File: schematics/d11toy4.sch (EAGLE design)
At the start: 15 parts, among them J1 usb, J2 strip, SW1 SPST_TACT-KMR2, U3 XC6206P332MR-G-SOT23

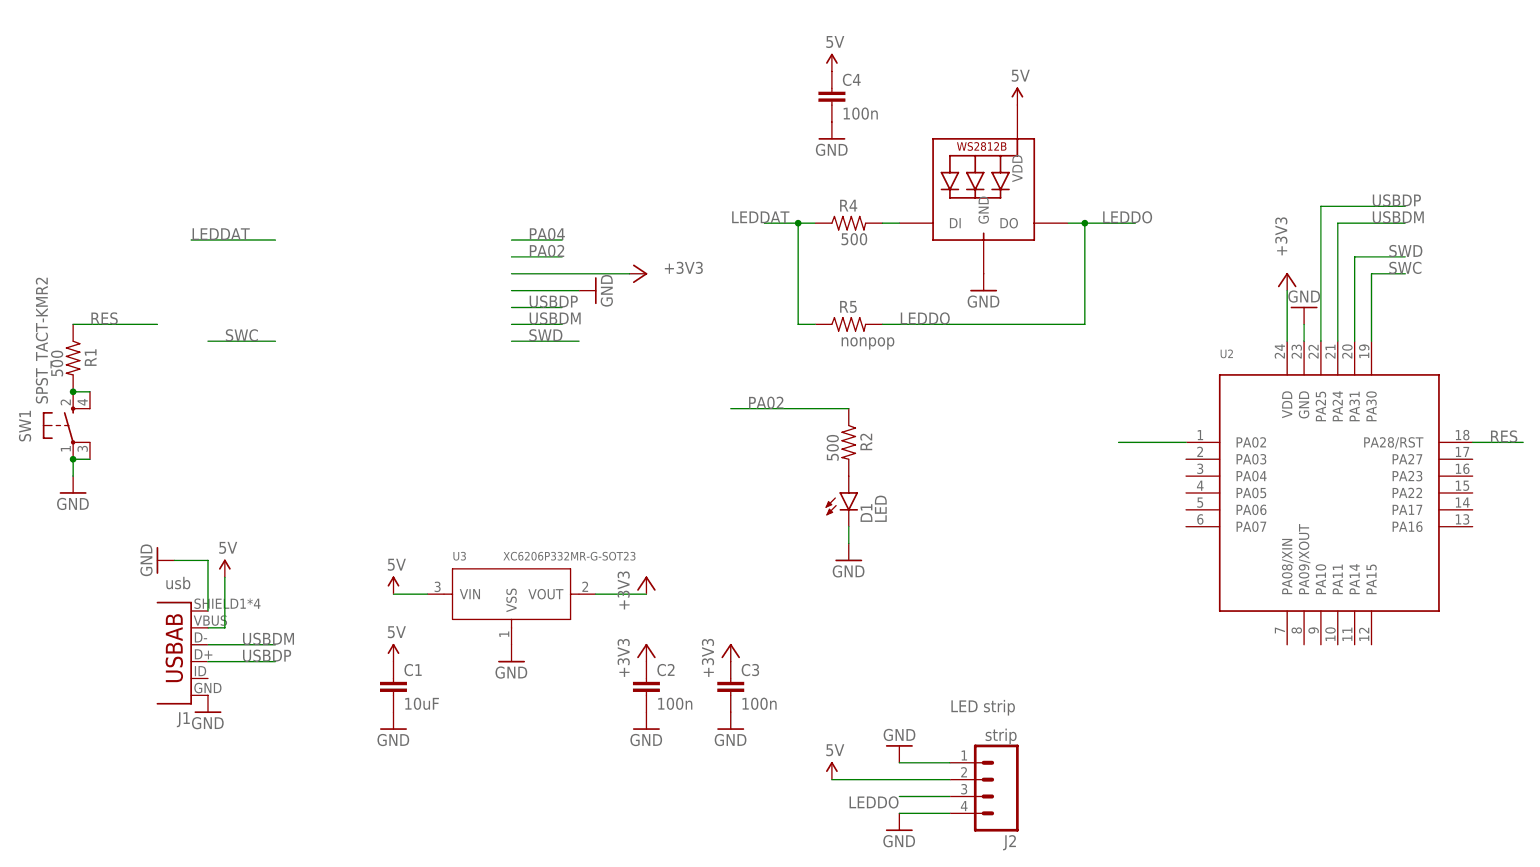
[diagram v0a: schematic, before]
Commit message: more experiments
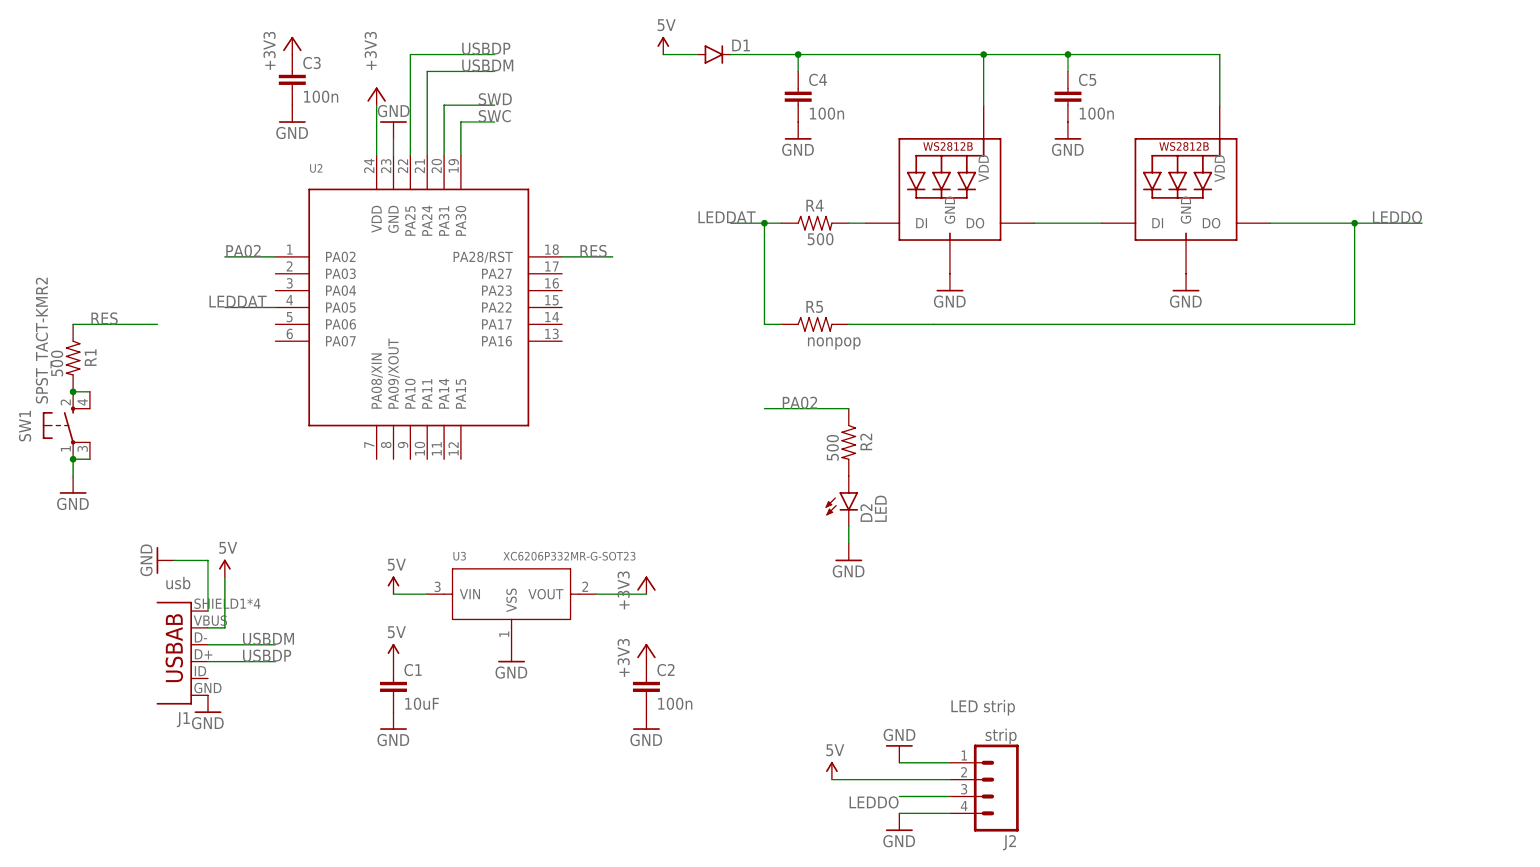
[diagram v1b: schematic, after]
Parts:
- added C5: 100n, SparkFun-Capacitors:CAP0603-CAP
- added D2: LED, SparkFun-LED:LED0603
- added LED2: WS2812B5050, adafruit:WS2812B5050
- D1: value LED -> (none); device SparkFun-LED:LED0603 -> SparkFun-DiscreteSemi:DIODESOD523
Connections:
- new net N$3: LED1.DO, LED2.DI
- new net N$4: C4.1, C5.1, D1.C, LED1.VDD, LED2.VDD
- net 5V: now also D1.A; no longer C4.1, LED1.VDD
- net GND: now also C5.2, D2.C, LED2.GND; no longer D1.C
- net LEDDAT: now also U2.PA05
- net LEDDO: now also LED2.DO; no longer LED1.DO
- net N$1: now also D2.A; no longer D1.A
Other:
- moved on the sheet: C3, C4, R4, R5, U2
